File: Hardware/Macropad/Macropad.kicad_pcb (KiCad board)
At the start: 4 copper layers, 80.5 x 57.5 mm, 53 parts, among them IC1 TLV77333PDBVR, J2 GSB1C41110SSHR, J3 Conn_01x04_Pin, J4 103R012BB100, Q1 BC847BS,115, U2 STM32F411C_C-E_Ux, Y2 ASDDV-16.000MHZ-LR-T

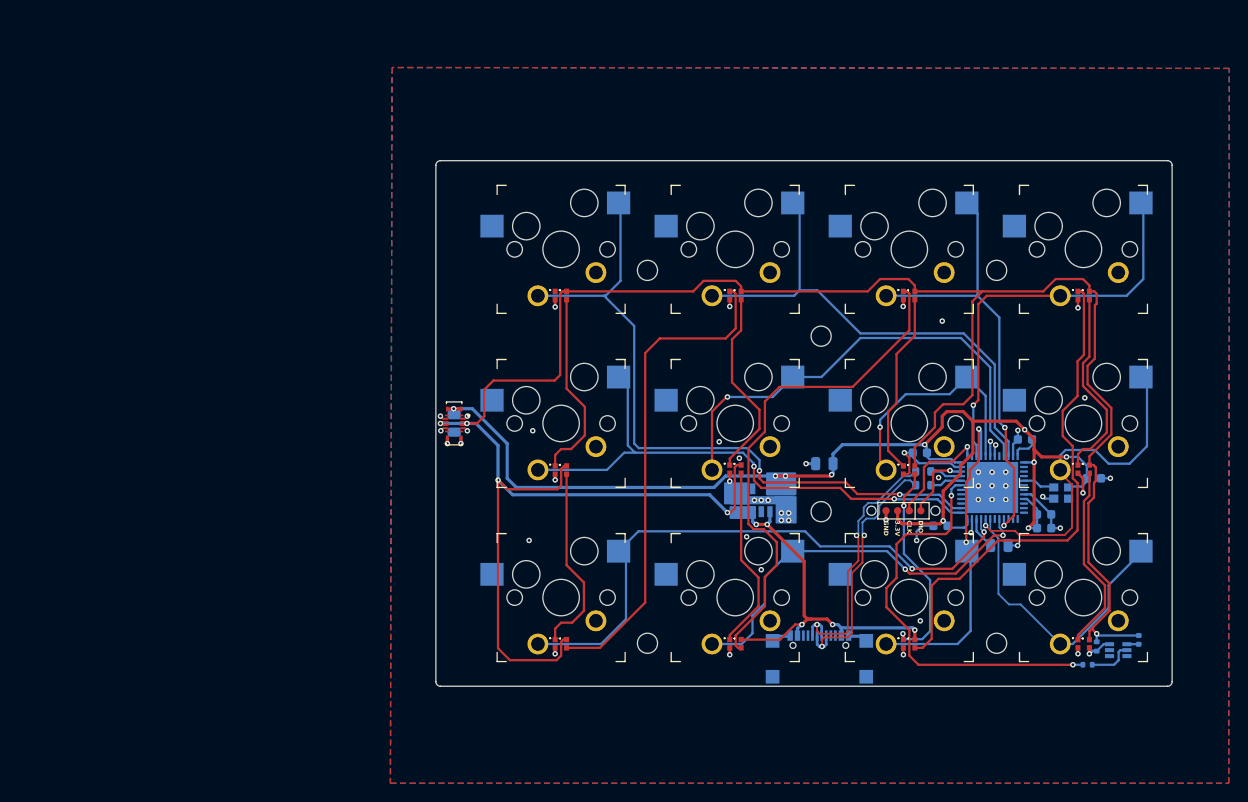
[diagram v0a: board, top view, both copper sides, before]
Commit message: Added Wheel
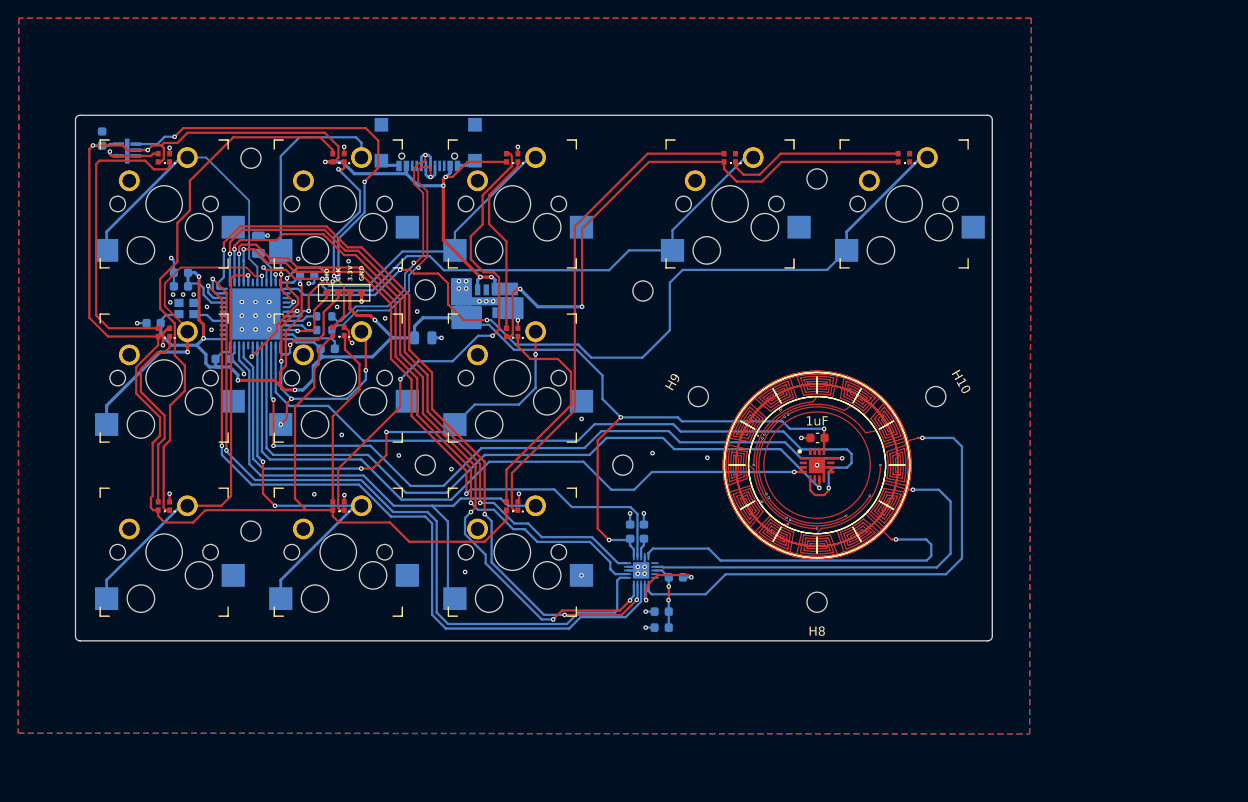
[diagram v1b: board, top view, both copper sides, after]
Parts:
- removed C16: 4.7uF, Capacitor_SMD:C_0805_2012Metric
- removed J4: 103R012BB100, 103R012BB100:AMPHENOL_103R012BB100
- removed LED12: WS2812B, XINGLIGHT XL-1515RGBC-WS2812B:XINGLIGHT XL-1515RGBC-WS2812B
- removed Q1: BC847BS,115, BC847BS:SOT65P210X110-6N
- removed R1: 2.2k, Resistor_SMD:R_0402_1005Metric
- removed R3: 10k, Resistor_SMD:R_0402_1005Metric
- removed S12: Keyswitch, MX Switches:Kailh_socket_MX_optional
- added C14: 100nF, Capacitor_SMD:C_0603_1608Metric, B.Cu at (163.5, 100.6)
- added C15: 100nF, Capacitor_SMD:C_0603_1608Metric, B.Cu at (160.1, 91.8)
- added C5: 1uF, Capacitor_SMD:C_0603_1608Metric, F.Cu at (180.6, 81.6)
- added C7: 100nF, Capacitor_SMD:C_0603_1608Metric, B.Cu at (165.1, 96.8)
- added C8: 10uF, Capacitor_SMD:C_0603_1608Metric, B.Cu at (163.5, 102.3)
- added C9: 100nF, Capacitor_SMD:C_0603_1608Metric, B.Cu at (161.6, 91.8)
- added H10: MountingHole, MountingHole:MountingHole_2.2mm_M2, F.Cu at (193.5, 77.1)
- added H7: MountingHole, MountingHole:MountingHole_2.2mm_M2, F.Cu at (180.5, 53.2)
- added H8: MountingHole, MountingHole:MountingHole_2.2mm_M2, F.Cu at (180.5, 99.6)
- added H9: MountingHole, MountingHole:MountingHole_2.2mm_M2, F.Cu at (167.5, 77.1)
- added IC2: MA702GQ-P, SamacSys_Parts:QFN50P300X300X100-17N-D, F.Cu at (180.5, 84.6)
- added IC3: SN74LV1T08DCKR, SamacSys_Parts:SOT65P210X110-5N, B.Cu at (105.0, 50.1)
- added IC4: TMC6300-LA, SamacSys_Parts:QFN40P300X300X90-21N, B.Cu at (161.3, 96.1)
- added NT1: NetTie_2, NetTie_Custom:NetTie-2_SMD_Pad0.25mm, F.Cu at (188.9, 92.7)
- added NT2: NetTie_2, NetTie_Custom:NetTie-2_SMD_Pad0.25mm, F.Cu at (190.8, 87.2)
- added NT3: NetTie_2, NetTie_Custom:NetTie-2_SMD_Pad0.25mm, F.Cu at (191.8, 81.6)
- C6: value 10nF -> 100nF; footprint Capacitor_SMD:C_0402_1005Metric -> Capacitor_SMD:C_0603_1608Metric
- moved C6 126.0 mm to (102.3, 48.8)
- moved LED1 113.9 mm to (109.0, 50.9), turned to 0 degrees
- moved S1 109.4 mm to (109.1, 56.0), turned to 0 degrees
- moved S3 105.9 mm to (109.1, 94.1), turned to 0 degrees
- moved C4 104.3 mm to (107.9, 69.0), turned to 0 degrees
- moved LED3 103.3 mm to (109.0, 89.0), turned to 0 degrees
- moved LED2 101.8 mm to (109.0, 70.0), turned to 0 degrees
- moved S2 100.7 mm to (109.1, 75.0), turned to 0 degrees
- moved C10 98.5 mm to (110.9, 63.5), turned to 0 degrees
- moved Y2 97.8 mm to (111.5, 67.4), turned to 0 degrees
- moved C11 97.7 mm to (110.9, 65.0), turned to 0 degrees
- moved H4 97.3 mm to (118.6, 51.0), turned to 180 degrees
- moved C19 88.2 mm to (115.5, 72.9), turned to 0 degrees
- moved C18 87.5 mm to (119.4, 60.4), turned to -90 degrees
- moved H3 86.4 mm to (118.6, 91.8), turned to 180 degrees
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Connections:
- C6 pad 1: +5V -> GND
- C6 pad 2: GND -> +5V
- LED11 pad 1: Net-(LED11-DO) -> unconnected-(LED11-DO-Pad1)
- U2 pad 10: TIM2_CH1 | Rotary 1 -> TMC_UH
- U2 pad 11: TIM2_CH2 | Rotary 2 -> TMC_UL
- U2 pad 12: unconnected-(U2-PA2-Pad12) -> TMC_VH
- U2 pad 13: unconnected-(U2-PA3-Pad13) -> TMC_VL
- U2 pad 14: unconnected-(U2-PA4-Pad14) -> TMC_WH
- U2 pad 15: unconnected-(U2-PA5-Pad15) -> TMC_WL
- U2 pad 16: switch 6 -> TMC_DIAG
- U2 pad 17: switch 7 -> switch 3
- U2 pad 18: unconnected-(U2-PB0-Pad18) -> ALED_Rotary
- U2 pad 29: unconnected-(U2-PA8-Pad29) -> switch 4
- U2 pad 30: unconnected-(U2-PA9-Pad30) -> switch 5
- U2 pad 38: unconnected-(U2-PA15-Pad38) -> SPI1_CS
- U2 pad 39: switch 3 -> SPI1_SCK
- U2 pad 40: switch 4 -> SPI1_MISO
- U2 pad 41: switch 5 -> SPI1_MOSI
- U2 pad 42: I2C1_SCL -> switch 6
- U2 pad 43: I2C1_SDA -> switch 7
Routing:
- net unconnected-(NT2-Pad2): track 0.00 -> 1068.0 mm, vias 0 -> 29
- net TMC_UH: track 0.00 -> 84.5 mm, vias 0 -> 2
- net TMC_VH: track 0.00 -> 83.8 mm, vias 0 -> 4
- net TMC_UL: track 0.00 -> 83.6 mm, vias 0 -> 2
- net SPI1_CS: track 0.00 -> 82.0 mm, vias 0 -> 1
- net TMC_WH: track 0.00 -> 80.5 mm, vias 0 -> 4
- net SPI1_SCK: track 0.00 -> 80.1 mm, vias 0 -> 3
- net SPI1_MISO: track 0.00 -> 79.5 mm, vias 0 -> 1
- net SPI1_MOSI: track 0.00 -> 76.8 mm, vias 0 -> 1
- net switch 12: track 75.4 -> 0.00 mm, vias 2 -> 0
- net I2C1_SDA: track 74.2 -> 0.00 mm, vias 3 -> 0
- net I2C1_SCL: track 74.2 -> 0.00 mm, vias 3 -> 0
- net TMC_VL: track 0.00 -> 71.9 mm, vias 0 -> 2
- net TMC_DIAG: track 0.00 -> 71.2 mm, vias 0 -> 2
- net TMC_WL: track 0.00 -> 69.9 mm, vias 0 -> 2
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- added copper zone on F.Cu, net (none)
- added copper zone on In1.Cu, net (none)
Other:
- board size 80.5 x 57.5 mm -> 100.3 x 57.5 mm
